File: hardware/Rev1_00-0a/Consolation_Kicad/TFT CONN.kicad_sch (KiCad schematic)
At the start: 42 parts, among them J3 62684-402100ALF, J9 5051101092, U26 TPS61169DCKR

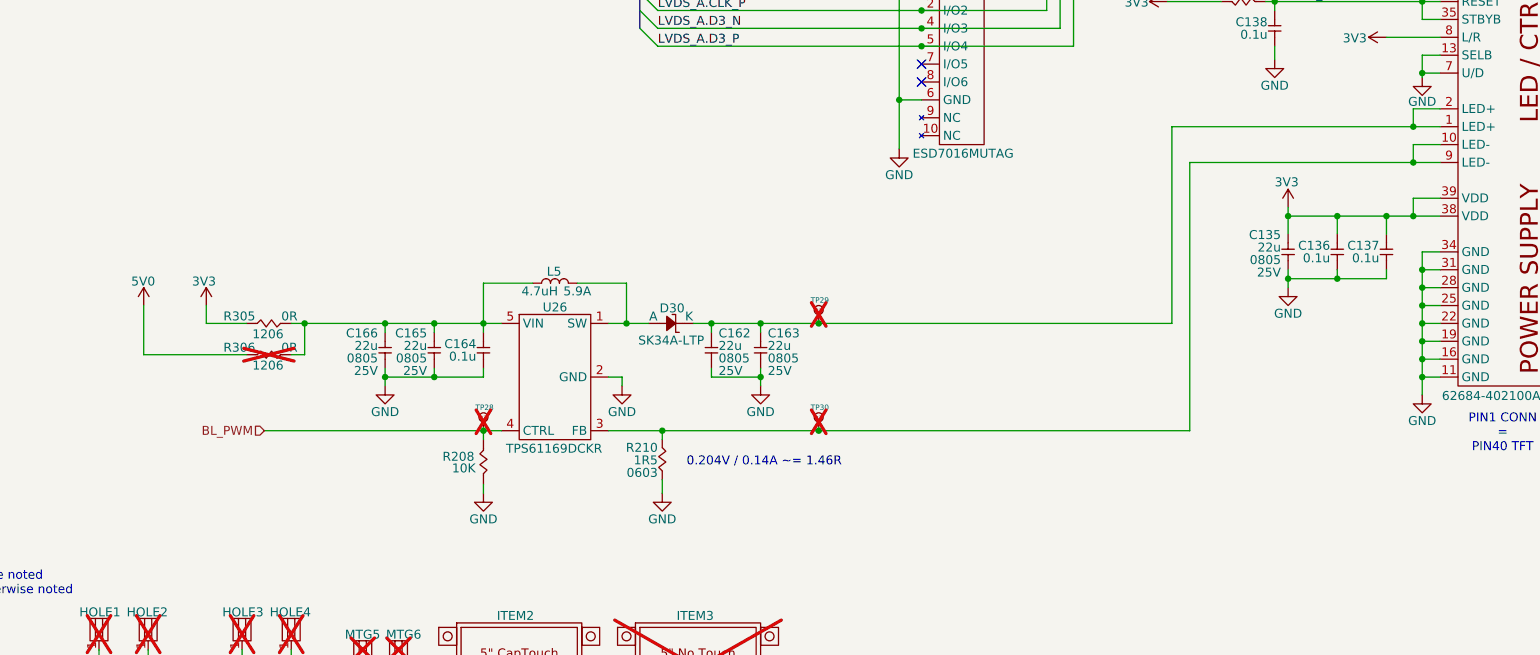
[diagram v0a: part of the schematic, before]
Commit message: Update PinMux & Schematics
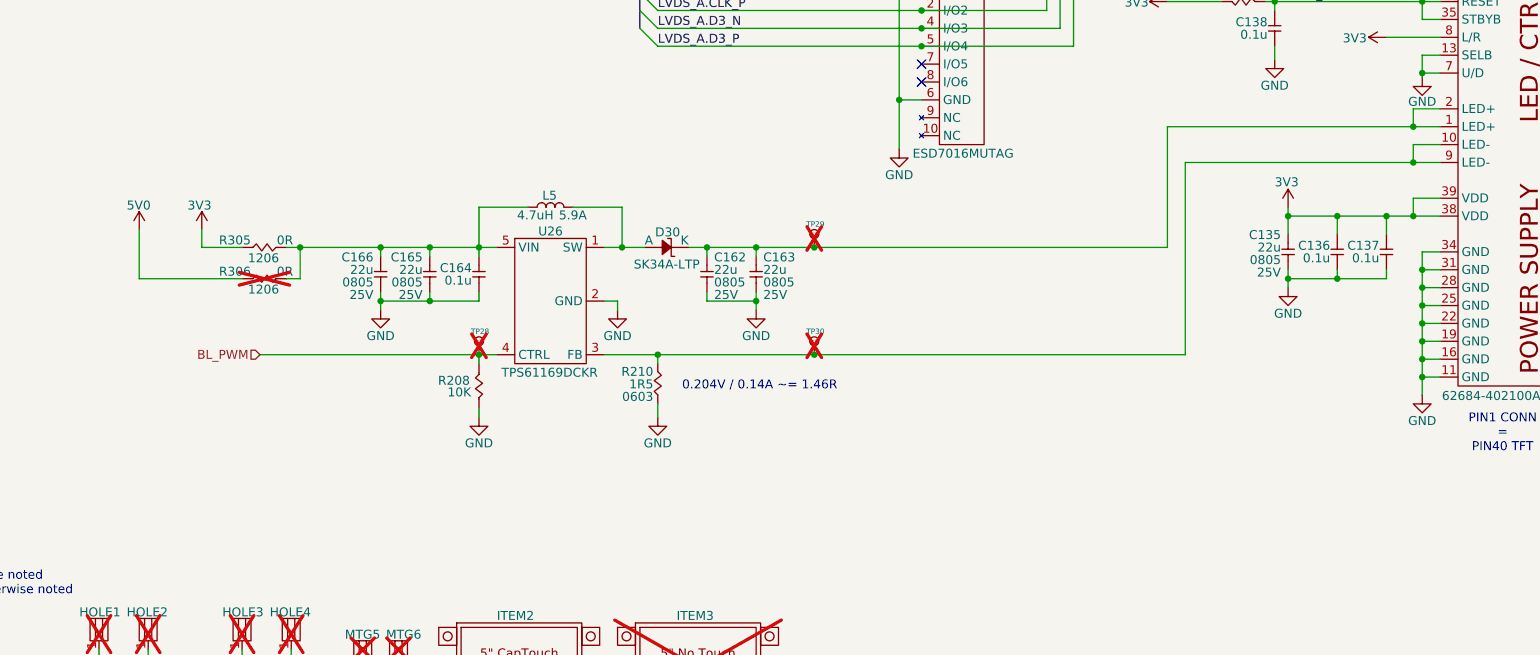
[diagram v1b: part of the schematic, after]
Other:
- moved on the sheet: C162, C163, C164, C165, C166, D30, L5, R208, R210, R305, R306, TP28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
